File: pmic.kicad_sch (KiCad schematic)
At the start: 18 parts, among them U3 STPMIC25APQR

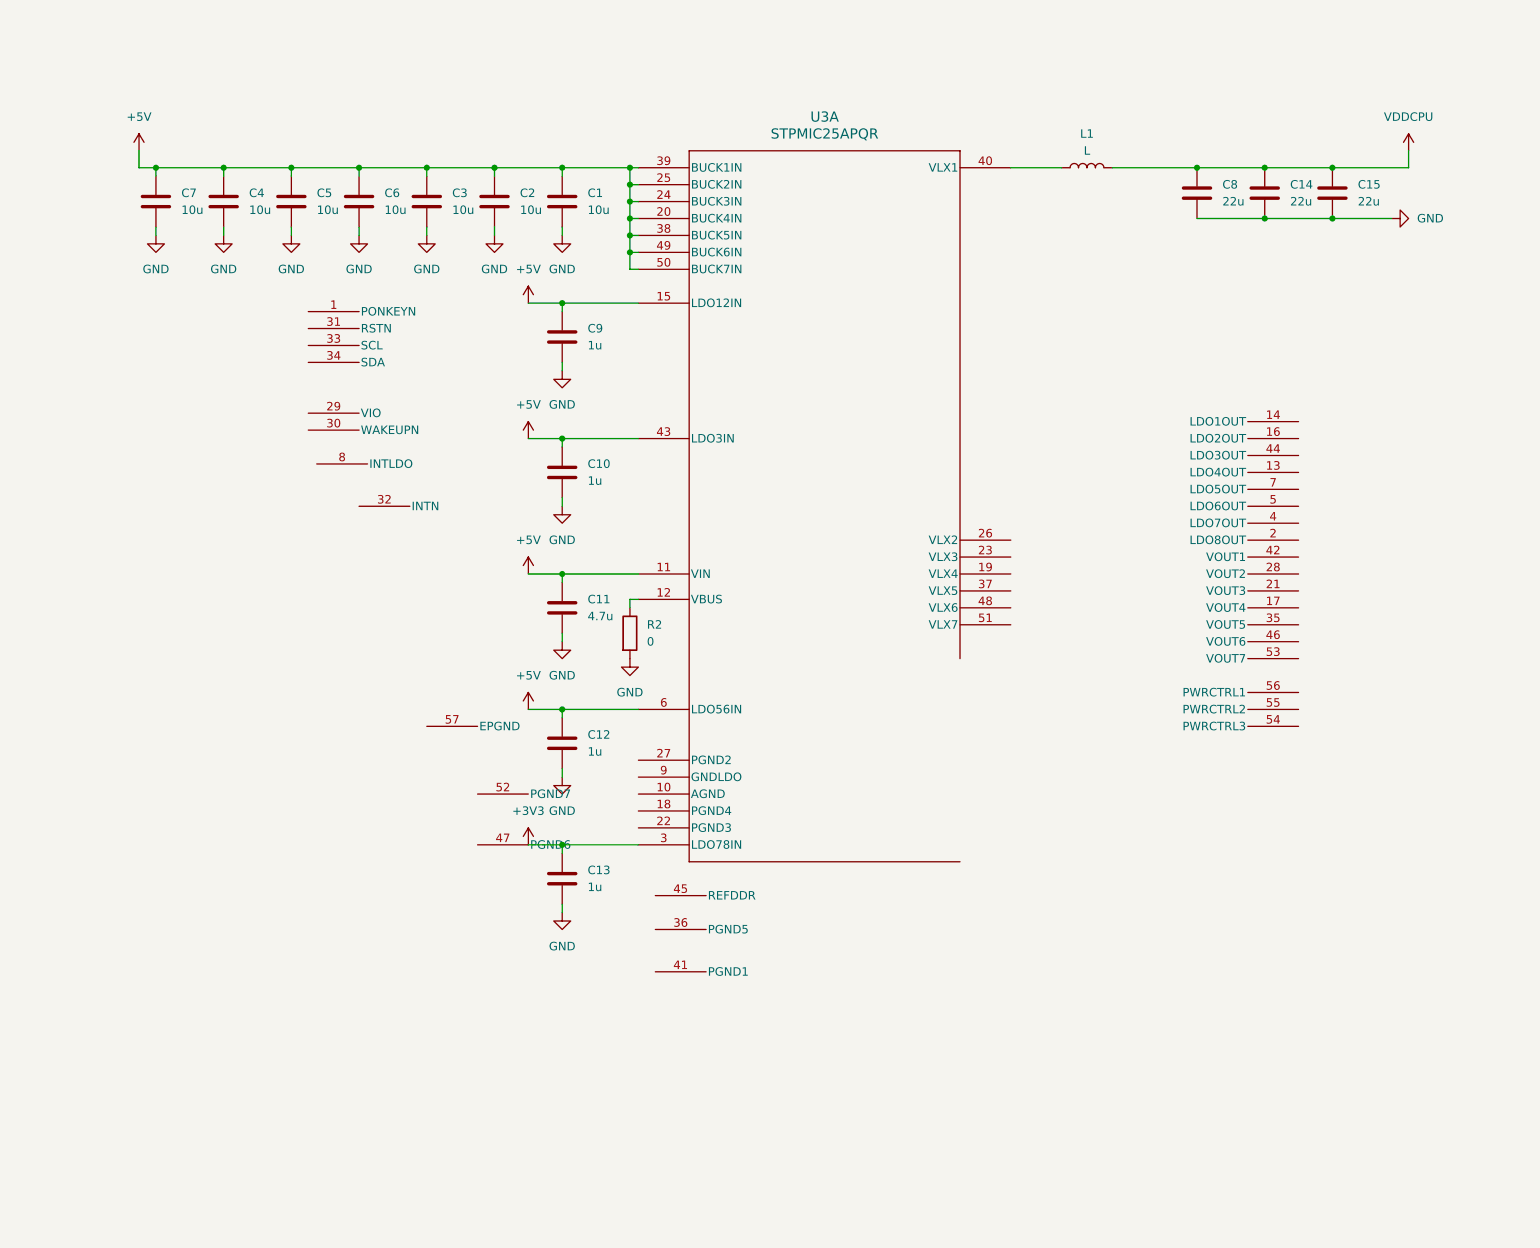
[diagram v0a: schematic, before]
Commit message: more pmic work
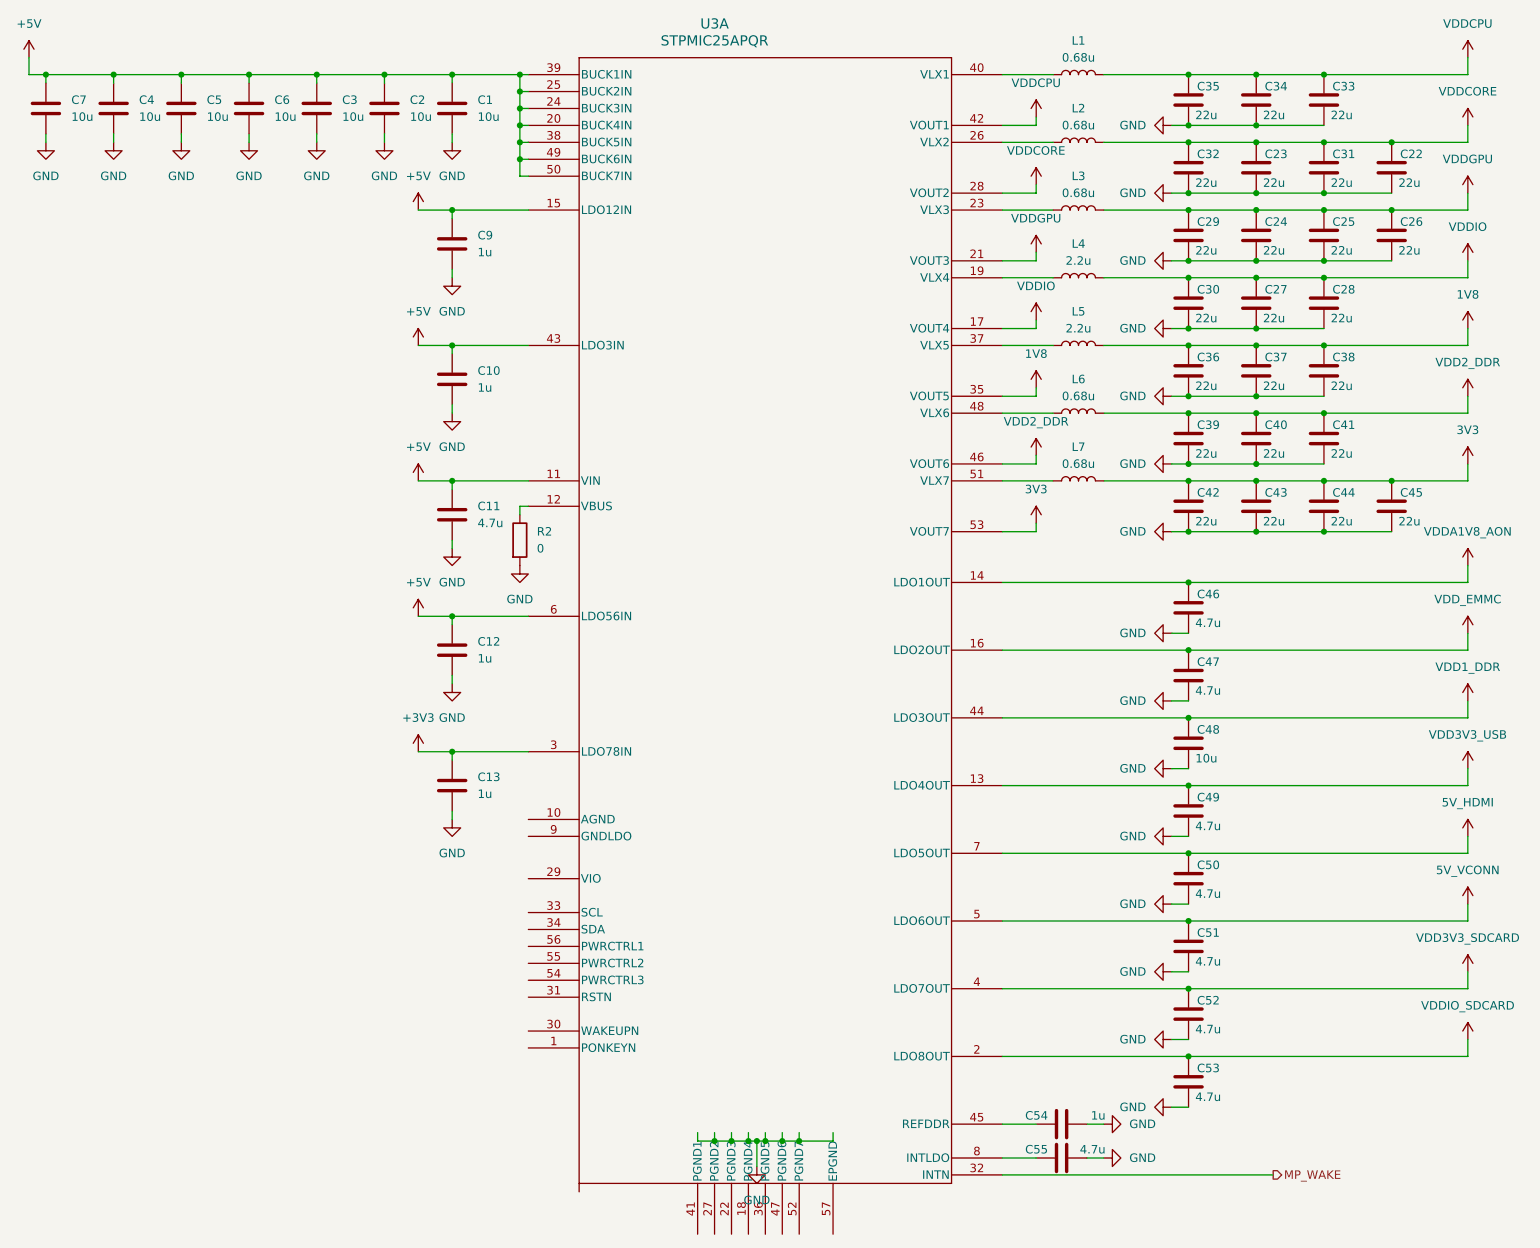
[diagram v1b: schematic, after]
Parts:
- removed C14, C15, C8: 22u, symbol Device:C
- added C22, C23, C24, C25, C26, C27, C28, C29, C30, C31, C32, C33, C34, C35, C36, C37, C38, C39, C40, C41, C42, C43, C44, C45: 22u, symbol Device:C
- added C46, C47, C49, C50, C51, C52, C53, C55: 4.7u, symbol Device:C
- added C48: 10u, symbol Device:C
- added C54: 1u, symbol Device:C
- added L2, L3, L6, L7: 0.68u, symbol Device:L
- added L4, L5: 2.2u, symbol Device:L
- L1: value L -> 0.68u
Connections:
- net GND: now also C22.1, C23.1, C24.1, C25.1, C26.1, C27.1, C28.1, C29.1, C30.1, C31.1, C32.1, C33.1, C34.1, C35.1, C36.1, C37.1, C38.1, C39.1, C40.1, C41.1, C42.1, C43.1, C44.1, C45.1, C46.1, C47.1, C48.1, C49.1, C50.1, C51.1, C52.1, C53.1, C54.1, C55.1
- net VDDCPU: now also U3.42 (VOUT1), C33.2, C34.2, C35.2
- net VDD3V3_USB: now reaches U3.13 (LDO4OUT)
- net VDD3V3_USB: now also C49.2
- net VDDA1V8_AON: now reaches U3.14 (LDO1OUT)
- net VDDA1V8_AON: now also C46.2
- net VDD_EMMC: now reaches U3.16 (LDO2OUT)
- net VDD_EMMC: now also C47.2
- net VDDIO: now reaches U3.17 (VOUT4)
- net VDDIO: now also C27.2, C28.2, C30.2, L4.2
- net at U3.19 (VLX4): now also L4.1
- net VDDIO_SDCARD: now reaches U3.2 (LDO8OUT)
- net VDDIO_SDCARD: now also C53.2
- net VDDGPU: now reaches U3.21 (VOUT3)
- net VDDGPU: now also C24.2, C25.2, C26.2, C29.2, L3.2
- net at U3.23 (VLX3): now also L3.1
- net at U3.26 (VLX2): now also L2.1
- net VDDCORE: now reaches U3.28 (VOUT2)
- net VDDCORE: now also C22.2, C23.2, C31.2, C32.2, L2.2
- net MP_WAKE: now reaches U3.32 (INTN)
- net 1V8: now reaches U3.35 (VOUT5)
- net 1V8: now also C36.2, C37.2, C38.2, L5.2
- net at U3.37 (VLX5): now also L5.1
- net VDD3V3_SDCARD: now reaches U3.4 (LDO7OUT)
- net VDD3V3_SDCARD: now also C52.2
- net VDD1_DDR: now reaches U3.44 (LDO3OUT)
- net VDD1_DDR: now also C48.2
- net at U3.45 (REFDDR): now also C54.2
- net VDD2_DDR: now reaches U3.46 (VOUT6)
- net VDD2_DDR: now also C39.2, C40.2, C41.2, L6.2
- net at U3.48 (VLX6): now also L6.1
- net 5V_VCONN: now reaches U3.5 (LDO6OUT)
- net 5V_VCONN: now also C51.2
- net at U3.51 (VLX7): now also L7.1
- net 3V3: now reaches U3.53 (VOUT7)
- net 3V3: now also C42.2, C43.2, C44.2, C45.2, L7.2
- net 5V_HDMI: now reaches U3.7 (LDO5OUT)
- net 5V_HDMI: now also C50.2
- net at U3.8 (INTLDO): now also C55.2
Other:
- moved on the sheet: C1, C10, C11, C12, C13, C2, C3, C4, C5, C6, C7, C9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
